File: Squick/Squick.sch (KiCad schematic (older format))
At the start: 30 parts

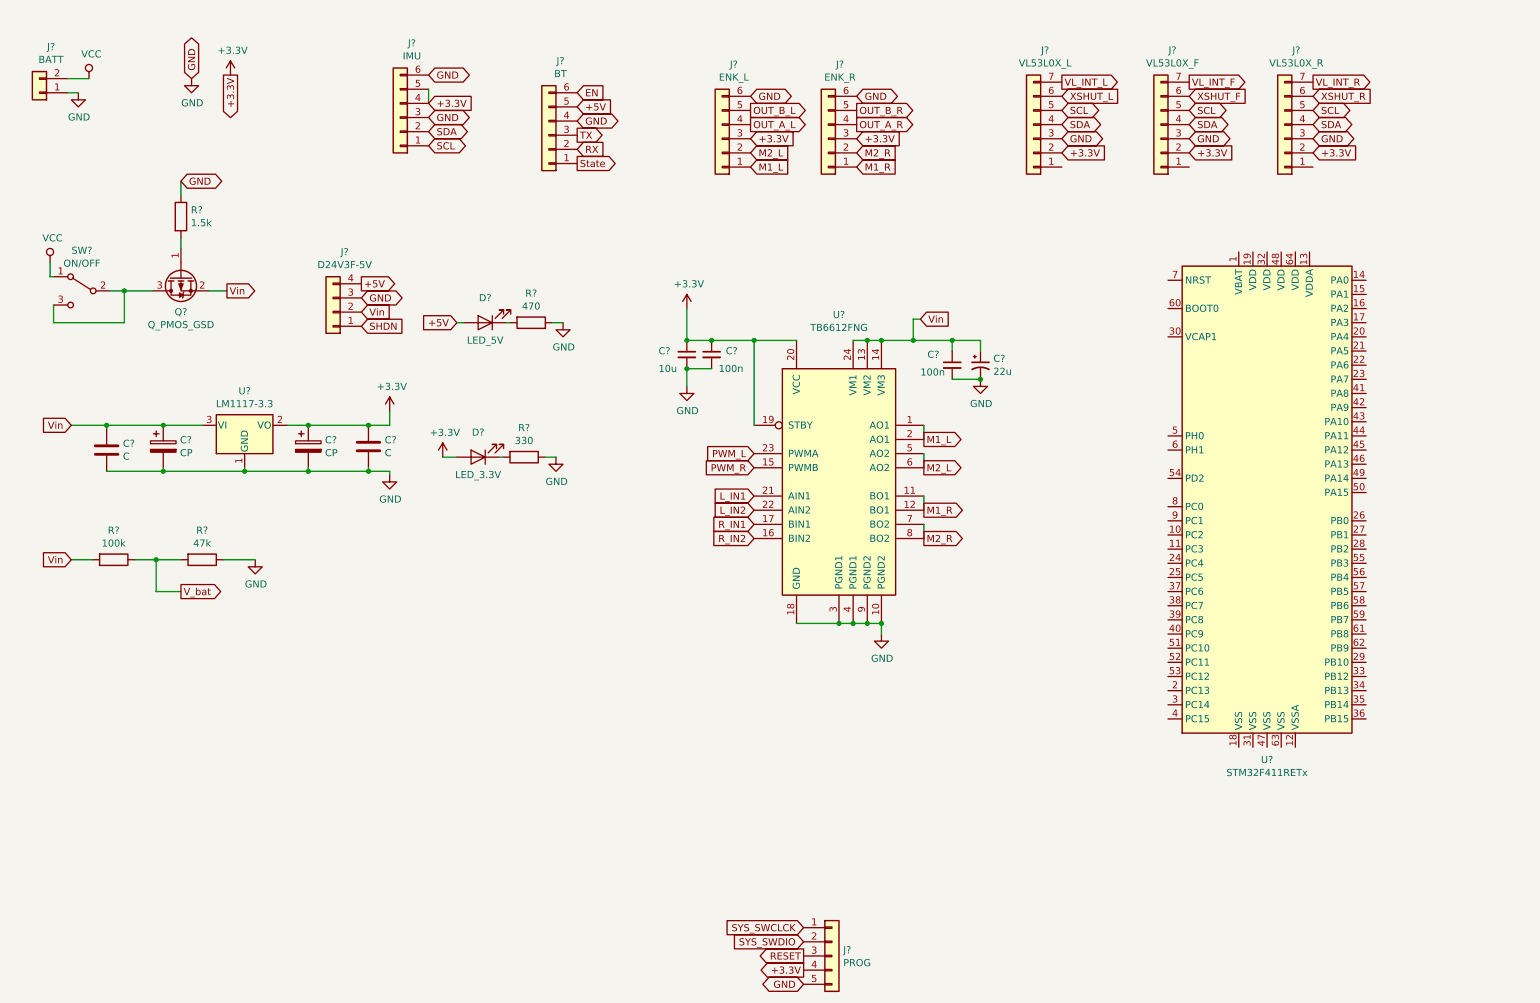
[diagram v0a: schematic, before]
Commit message: New progress in work
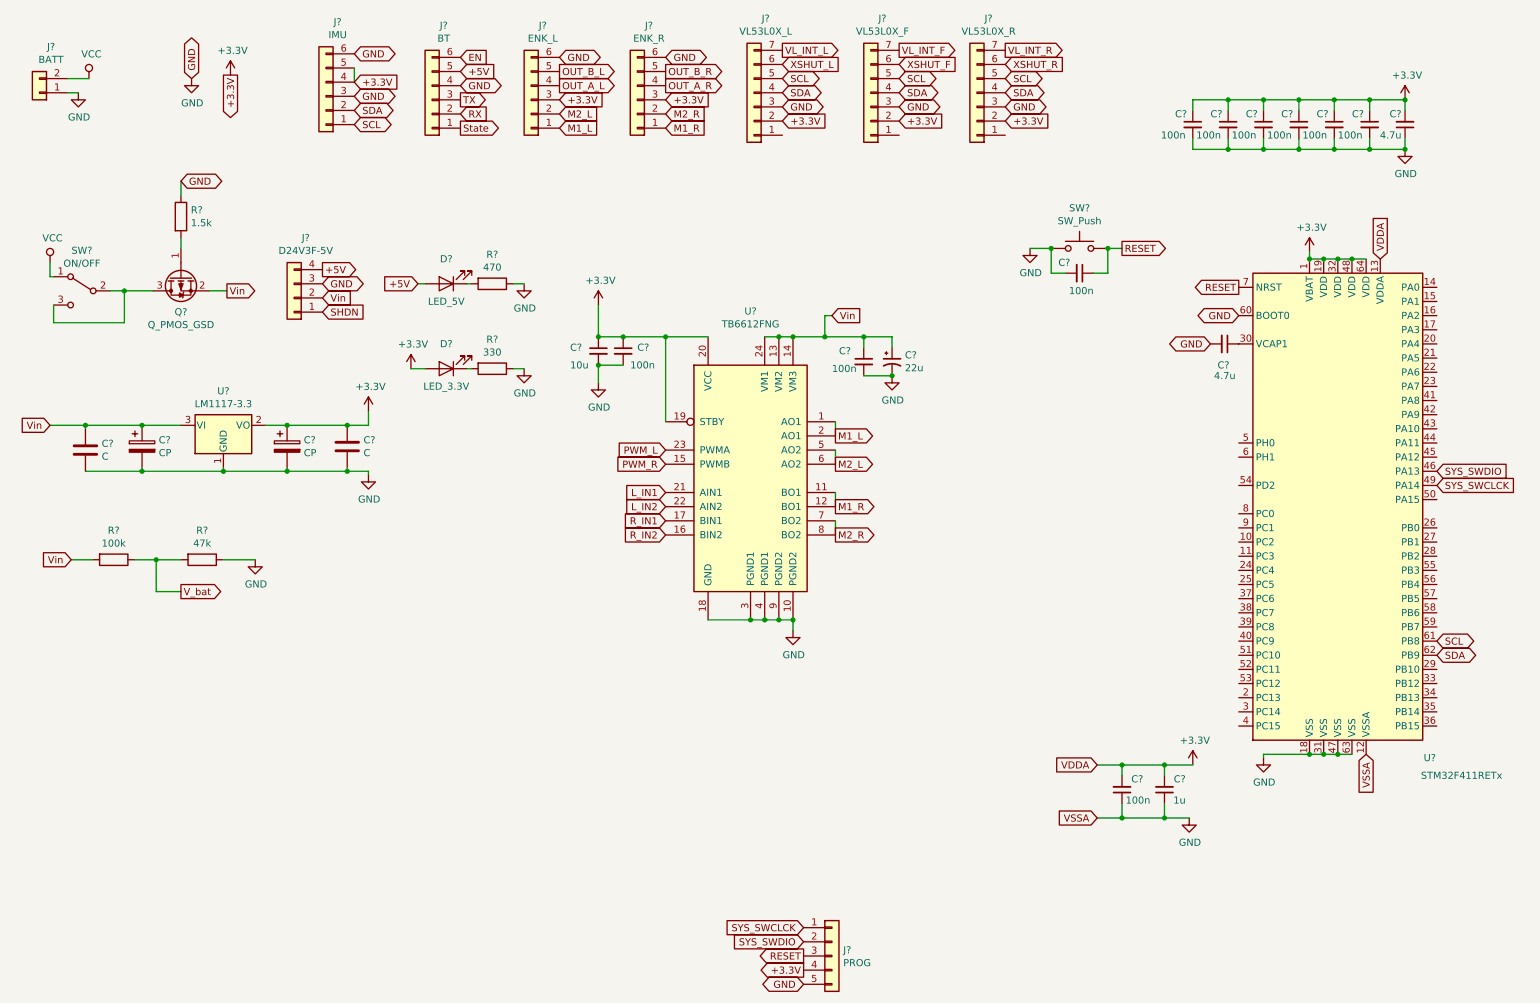
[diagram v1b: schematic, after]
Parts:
- added C? (x2): 4.7u, symbol Device:C_Small
- added C? (x8): 100n, symbol Device:C_Small
- added C?: 1u, symbol Device:C_Small
- added SW?: SW_Push, symbol Switch:SW_Push
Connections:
- net +3V3: now also U?.1 (VBAT), U?.13 (VDDA), U?.19 (VDD), U?.32 (VDD), U?.48 (VDD), U?.64 (VDD), C?.1, C?.1, C?.1, C?.1, C?.1, C?.1, C?.2, C?.2, C?.2
- net GND: now also U?.12 (VSSA), U?.18 (VSS), U?.31 (VSS), U?.47 (VSS), U?.60 (BOOT0), U?.63 (VSS), C?.1, C?.1, C?.1, C?.2, C?.2, C?.2, C?.2, C?.2, C?.2, C?.2, C?.2, SW?.1
- net RESET: now also U?.7 (NRST), C?.1, SW?.2
- net SCL: now also U?.61 (PB8)
- net SDA: now also U?.62 (PB9)
- net SYS_SWCLCK: now also U?.49 (PA14)
- net SYS_SWDIO: now also U?.46 (PA13)
- net at U?.30 (VCAP1): now also C?.1
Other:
- moved on the sheet: C?, D?, J?, R?, U?

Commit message: End for today. Almost finished
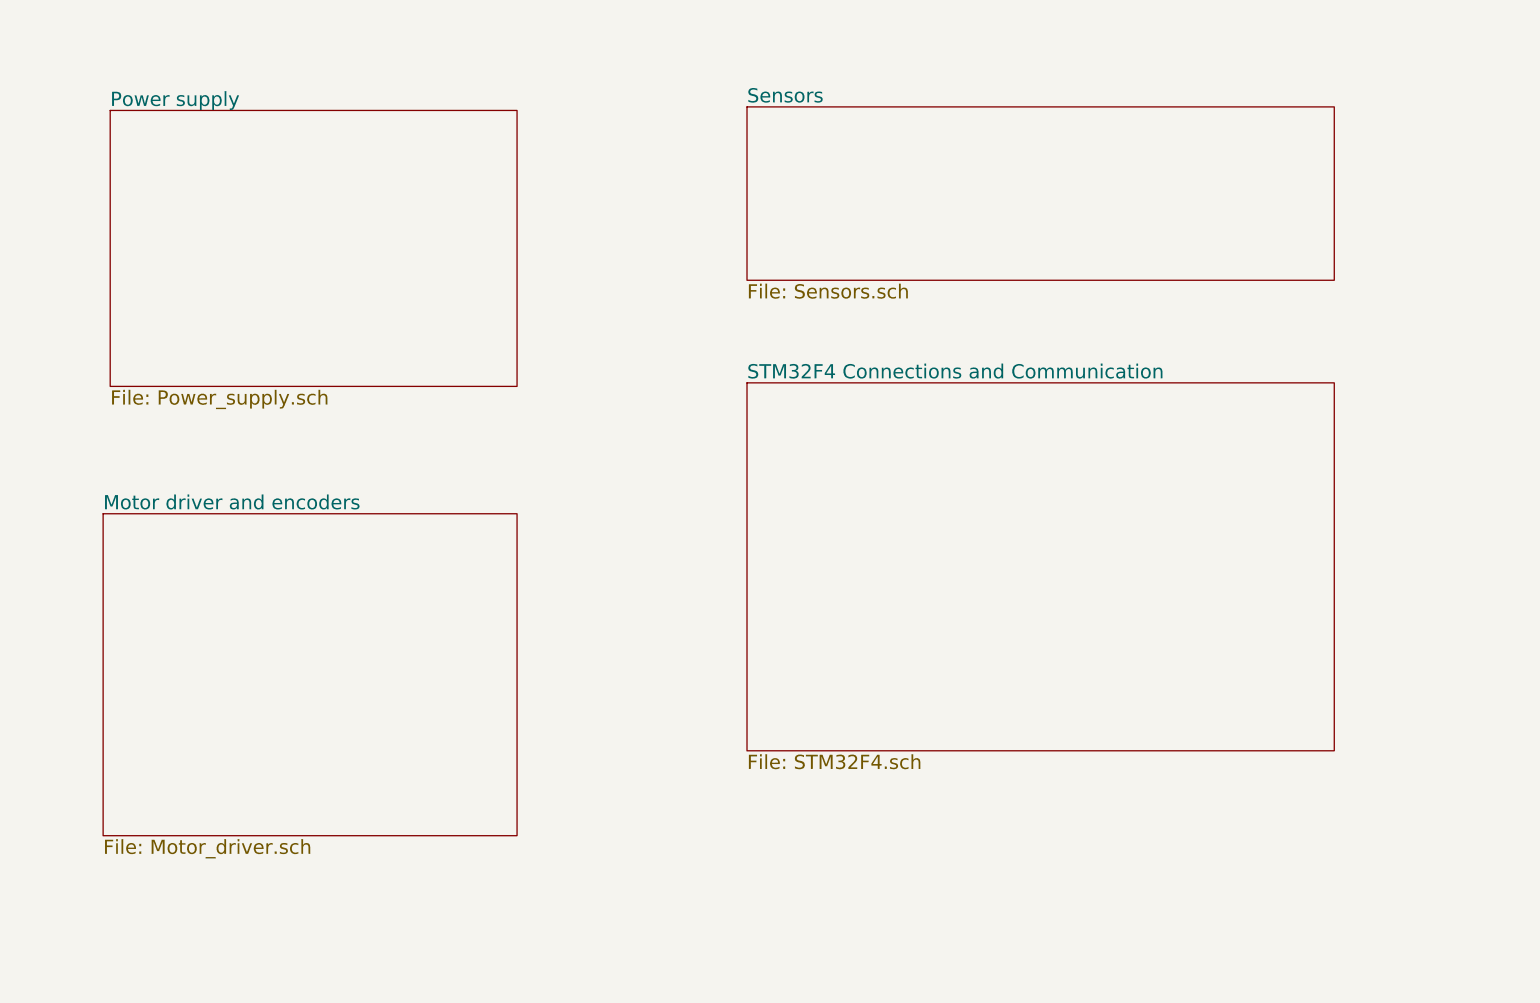
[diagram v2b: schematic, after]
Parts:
- removed C?: 22u, symbol Device:CP1_Small
- removed C? (x10): 100n, symbol Device:C_Small
- removed C?: 10u, symbol Device:C_Small
- removed C? (x2): 4.7u, symbol Device:C_Small
- removed C? (x2): C, symbol Device:C
- removed C? (x2): CP, symbol Device:CP
- removed C?: 1u, symbol Device:C_Small
- removed D?: LED_3.3V, symbol Device:LED
- removed D?: LED_5V, symbol Device:LED
- removed J?: D24V3F-5V, symbol Connector_Generic:Conn_01x04
- removed J?: BT, symbol Connector_Generic:Conn_01x06
- removed J?: VL53L0X_L, symbol Connector_Generic:Conn_01x07
- removed J?: VL53L0X_F, symbol Connector_Generic:Conn_01x07
- removed J?: VL53L0X_R, symbol Connector_Generic:Conn_01x07
- removed J?: ENK_L, symbol Connector_Generic:Conn_01x06
- removed J?: ENK_R, symbol Connector_Generic:Conn_01x06
- removed J?: IMU, symbol Connector_Generic:Conn_01x06
- removed J?: BATT, symbol Connector_Generic:Conn_01x02
- removed J?: PROG, symbol Connector_Generic:Conn_01x05
- removed Q?: Q_PMOS_GSD, symbol Device:Q_PMOS_GSD
- removed R?: 1.5k, symbol Device:R
- removed R?: 100k, symbol Device:R
- removed R?: 47k, symbol Device:R
- removed R?: 330, symbol Device:R
- removed R?: 470, symbol Device:R
- removed SW?: ON/OFF, symbol Switch:SW_SPDT
- removed SW?: SW_Push, symbol Switch:SW_Push
- removed U?: STM32F411RETx, Package_QFP:LQFP-64_10x10mm_P0.5mm, symbol MCU_ST_STM32F4:STM32F411RETx
- removed U?: TB6612FNG, Package_SO:SSOP-24_5.3x8.2mm_P0.65mm, symbol Driver_Motor:TB6612FNG
- removed U?: LM1117-3.3, symbol Regulator_Linear:LM1117-3.3
